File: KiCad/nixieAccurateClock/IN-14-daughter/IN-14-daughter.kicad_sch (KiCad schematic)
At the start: 6 parts, among them J1 Conn_02x11_Top_Bottom, U1 HV509K6-G

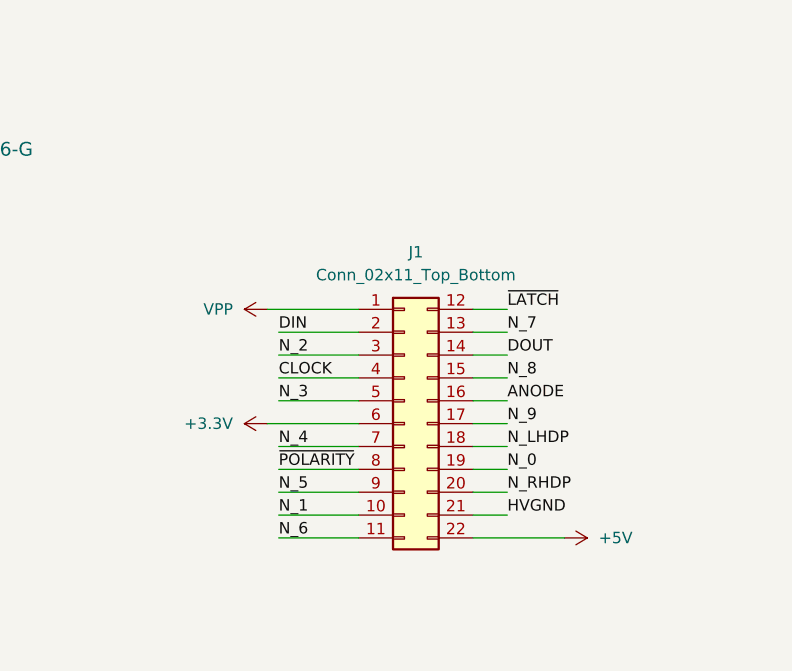
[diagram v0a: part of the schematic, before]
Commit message: reroute daughter board
Swapped standoffs and pin header orientation on IN-14 daughter board so that standoffs face outward.  This allows using the daughter board mounting for the mother board mounting.
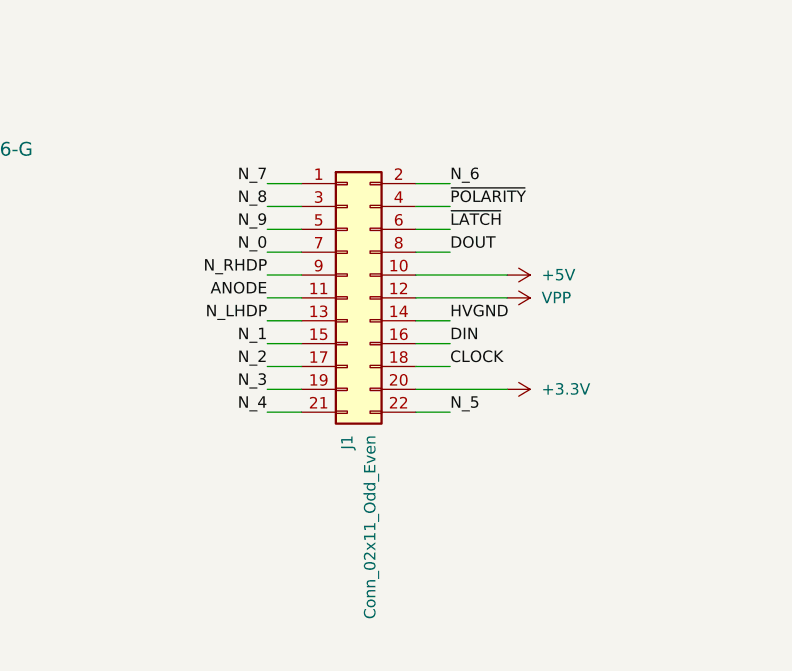
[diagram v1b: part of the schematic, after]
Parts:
- removed J1: Conn_02x11_Top_Bottom, Connector_PinHeader_1.27mm:PinHeader_2x11_P1.27mm_Vertical, symbol Connector_Generic:Conn_02x11_Top_Bottom
- added J1: Conn_02x11_Odd_Even, Connector_PinHeader_1.27mm:PinHeader_2x11_P1.27mm_Vertical, symbol Connector_Generic:Conn_02x11_Odd_Even
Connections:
- net +3.3V: now also J1.20 (Pin_20)
- net +5V: now also J1.10 (Pin_10)
- net ANODE: now also J1.11 (Pin_11)
- net CLOCK: now also J1.18 (Pin_18)
- net DIN: now also J1.16 (Pin_16)
- net DOUT: now also J1.8 (Pin_8)
- net HVGND: now also J1.14 (Pin_14)
- net N_0: now also J1.7 (Pin_7)
- net N_1: now also J1.15 (Pin_15)
- net N_2: now also J1.17 (Pin_17)
- net N_3: now also J1.19 (Pin_19)
- net N_4: now also J1.21 (Pin_21)
- net N_5: now also J1.22 (Pin_22)
- net N_6: now also J1.2 (Pin_2)
- net N_7: now also J1.1 (Pin_1)
- net N_8: now also J1.3 (Pin_3)
- net N_9: now also J1.5 (Pin_5)
- net N_LHDP: now also J1.13 (Pin_13)
- net N_RHDP: now also J1.9 (Pin_9)
- net VPP: now also J1.12 (Pin_12)
- net ~{LATCH}: now also J1.6 (Pin_6)
- net ~{POLARITY}: now also J1.4 (Pin_4)

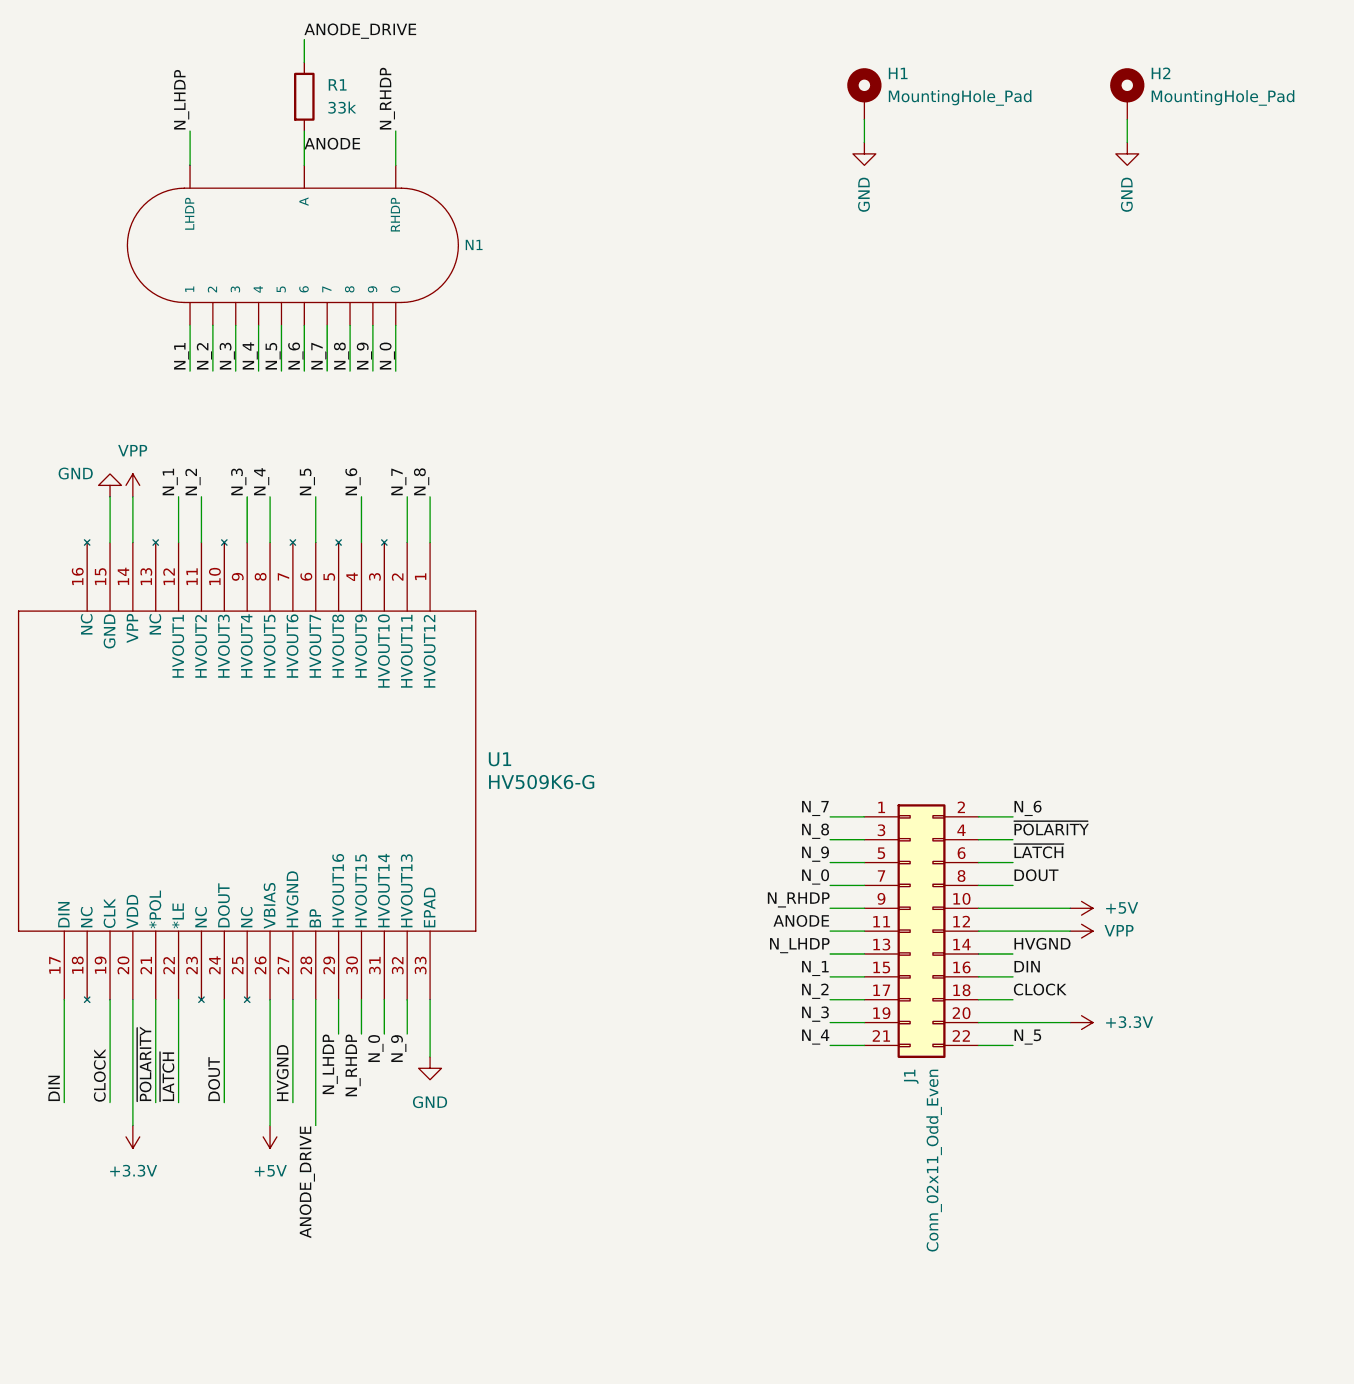
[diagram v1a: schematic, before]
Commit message: simplify nixie daughter board
Remove cathode pins that would not be usable for current sensing anyway.
Pivot to using anode pin as shunt measurement with a R2R flash ADC (not yet implemented).
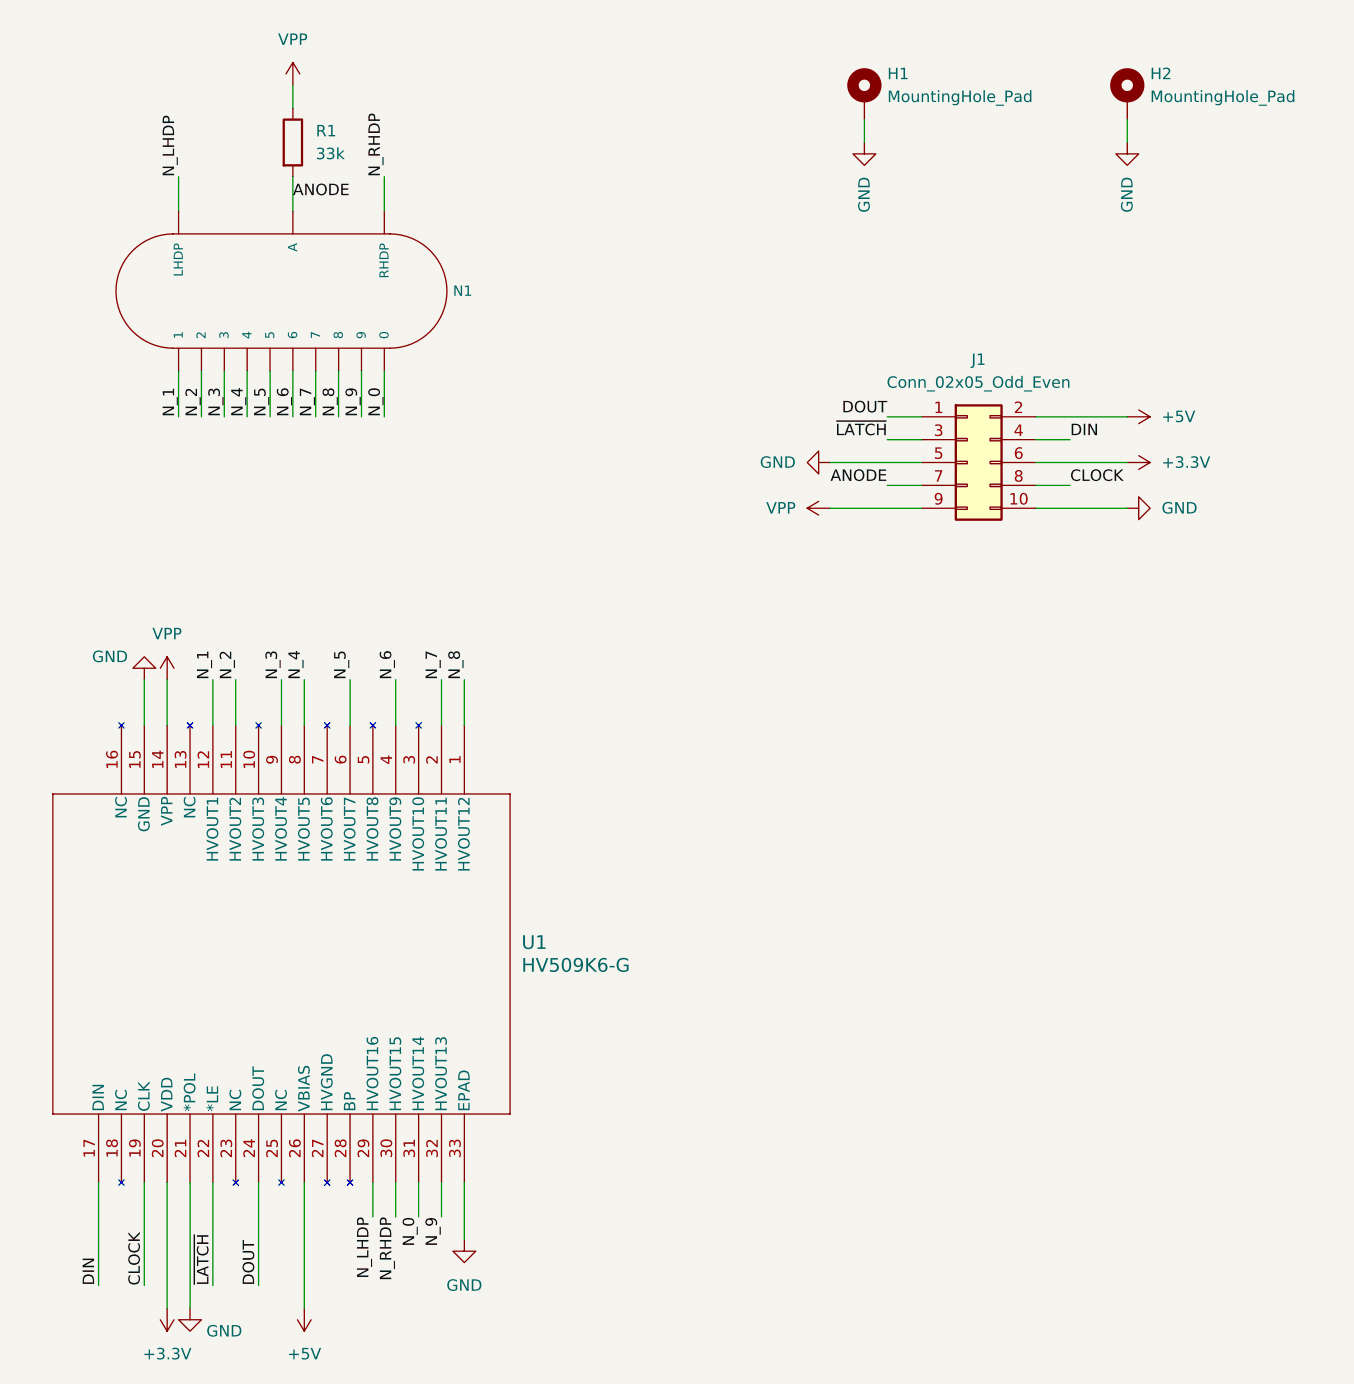
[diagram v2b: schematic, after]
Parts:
- removed J1: Conn_02x11_Odd_Even, Connector_PinHeader_1.27mm:PinHeader_2x11_P1.27mm_Vertical, symbol Connector_Generic:Conn_02x11_Odd_Even
- added J1: Conn_02x05_Odd_Even, Connector_PinHeader_2.54mm:PinHeader_2x05_P2.54mm_Vertical, symbol Connector_Generic:Conn_02x05_Odd_Even
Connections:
- net ~{POLARITY} is gone; now on net GND: U1.21 (*POL)
- net +3.3V: now also J1.6 (Pin_6)
- net +5V: now also J1.2 (Pin_2)
- net ANODE: now also J1.7 (Pin_7)
- net CLOCK: now also J1.8 (Pin_8)
- net DIN: now also J1.4 (Pin_4)
- net DOUT: now also J1.1 (Pin_1)
- net GND: now also J1.10 (Pin_10), J1.5 (Pin_5)
- net VPP: now also R1.1, J1.9 (Pin_9)
- net ~{LATCH}: now also J1.3 (Pin_3)
- net ANODE_DRIVE: no longer names the net of U1.28 (BP)
- net ANODE_DRIVE: no longer R1.1
- net HVGND: no longer names the net of U1.27 (HVGND)
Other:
- moved on the sheet: N1, R1

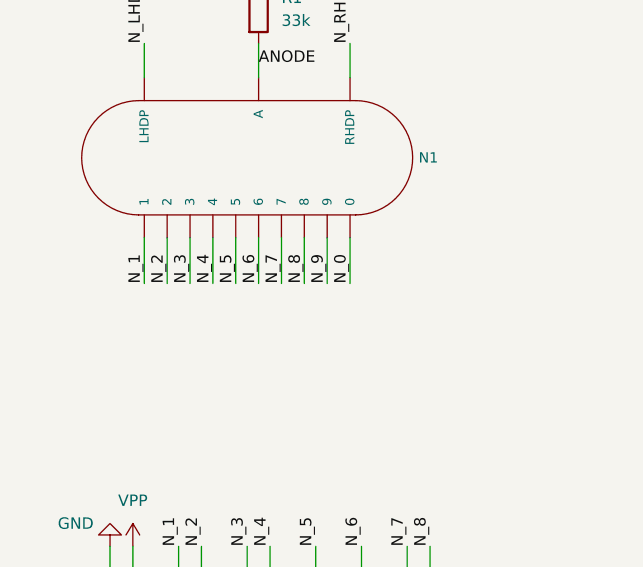
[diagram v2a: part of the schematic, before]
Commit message: fix clearance rules on daughter board
0.4 mm clearance is not possible to obey with an HV driver IC package that has 0.25 mm pad spacing, but all HV lines can be kept at least 0.25 mm away from everything else and inner layers can be preferentially used.

WIP ADC interface, logic level convertor has been chosen.
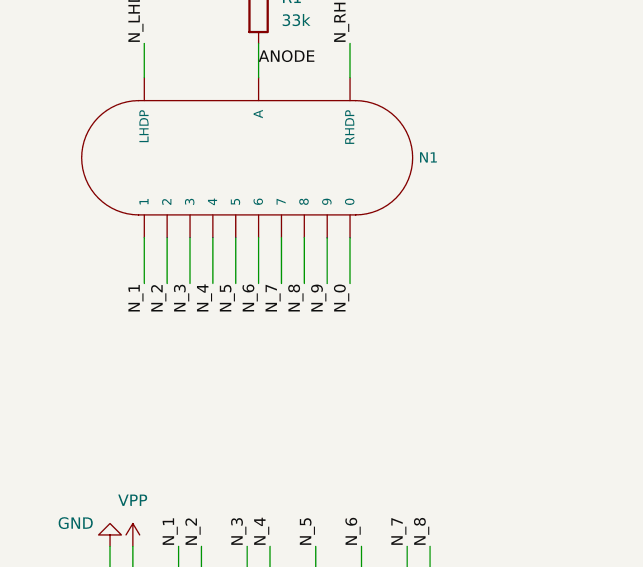
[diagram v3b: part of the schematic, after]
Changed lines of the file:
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@@
   (title_block
     (title "IN-14 daughter board")
+    (rev "A")
   )
   (wire (pts (xy 57.15 88.9) (xy 57.15 93.98))
@@
     (effects (font (size 1.27 1.27)) (justify right bottom))
   )
-  (label "N_2" (at 63.5 59.69 90) (fields_autoplaced)
-    (effects (font (size 1.27 1.27)) (justify left bottom))
+  (label "N_2" (at 63.5 59.69 270) (fields_autoplaced)
+    (effects (font (size 1.27 1.27)) (justify right bottom))
   )
   (label "DOUT" (at 139.7 59.69 180) (fields_autoplaced)
     (effects (font (size 1.27 1.27)) (justify right bottom))
   )
-  (label "N_4" (at 68.58 59.69 90) (fields_autoplaced)
-    (effects (font (size 1.27 1.27)) (justify left bottom))
+  (label "N_4" (at 68.58 59.69 270) (fields_autoplaced)
+    (effects (font (size 1.27 1.27)) (justify right bottom))
   )
   (label "DIN" (at 52.07 156.21 90) (fields_autoplaced)
     (effects (font (size 1.27 1.27)) (justify left bottom))
   )
-  (label "N_1" (at 60.96 59.69 90) (fields_autoplaced)
-    (effects (font (size 1.27 1.27)) (justify left bottom))
+  (label "N_1" (at 60.96 59.69 270) (fields_autoplaced)
+    (effects (font (size 1.27 1.27)) (justify right bottom))
   )
   (label "ANODE" (at 139.7 67.31 180) (fields_autoplaced)
@@
     (effects (font (size 1.27 1.27)) (justify left bottom))
   )
-  (label "N_3" (at 66.04 59.69 90) (fields_autoplaced)
-    (effects (font (size 1.27 1.27)) (justify left bottom))
+  (label "N_3" (at 66.04 59.69 270) (fields_autoplaced)
+    (effects (font (size 1.27 1.27)) (justify right bottom))
   )
   (label "N_3" (at 72.39 88.9 90) (fields_autoplaced)
@@
     (effects (font (size 1.27 1.27)) (justify right bottom))
   )
-  (label "N_5" (at 71.12 59.69 90) (fields_autoplaced)
-    (effects (font (size 1.27 1.27)) (justify left bottom))
+  (label "N_5" (at 71.12 59.69 270) (fields_autoplaced)
+    (effects (font (size 1.27 1.27)) (justify right bottom))
   )
   (label "N_1" (at 64.77 88.9 90) (fields_autoplaced)
@@
     (effects (font (size 1.27 1.27)) (justify left bottom))
   )
-  (label "N_9" (at 81.28 59.69 90) (fields_autoplaced)
-    (effects (font (size 1.27 1.27)) (justify left bottom))
+  (label "N_9" (at 81.28 59.69 270) (fields_autoplaced)
+    (effects (font (size 1.27 1.27)) (justify right bottom))
   )
   (label "CLOCK" (at 57.15 156.21 90) (fields_autoplaced)
@@
     (effects (font (size 1.27 1.27)) (justify left bottom))
   )
-  (label "N_7" (at 76.2 59.69 90) (fields_autoplaced)
-    (effects (font (size 1.27 1.27)) (justify left bottom))
+  (label "N_7" (at 76.2 59.69 270) (fields_autoplaced)
+    (effects (font (size 1.27 1.27)) (justify right bottom))
   )
   (label "N_LHDP" (at 60.96 33.02 90) (fields_autoplaced)
     (effects (font (size 1.27 1.27)) (justify left bottom))
   )
-  (label "N_8" (at 78.74 59.69 90) (fields_autoplaced)
-    (effects (font (size 1.27 1.27)) (justify left bottom))
+  (label "N_8" (at 78.74 59.69 270) (fields_autoplaced)
+    (effects (font (size 1.27 1.27)) (justify right bottom))
   )
   (label "N_LHDP" (at 82.55 148.59 270) (fields_autoplaced)
@@
     (effects (font (size 1.27 1.27)) (justify left bottom))
   )
-  (label "N_6" (at 73.66 59.69 90) (fields_autoplaced)
-    (effects (font (size 1.27 1.27)) (justify left bottom))
+  (label "N_6" (at 73.66 59.69 270) (fields_autoplaced)
+    (effects (font (size 1.27 1.27)) (justify right bottom))
   )
   (label "N_RHDP" (at 83.82 33.02 90) (fields_autoplaced)
@@
     (effects (font (size 1.27 1.27)) (justify left bottom))
   )
-  (label "N_0" (at 83.82 59.69 90) (fields_autoplaced)
-    (effects (font (size 1.27 1.27)) (justify left bottom))
+  (label "N_0" (at 83.82 59.69 270) (fields_autoplaced)
+    (effects (font (size 1.27 1.27)) (justify right bottom))
   )
   (symbol (lib_id "power:GND") (at 137.16 29.21 0) (mirror y) (unit 1)
